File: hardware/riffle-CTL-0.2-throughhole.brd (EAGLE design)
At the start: 36.8 x 18 mm, 14 parts, among them J2 AYZ0202

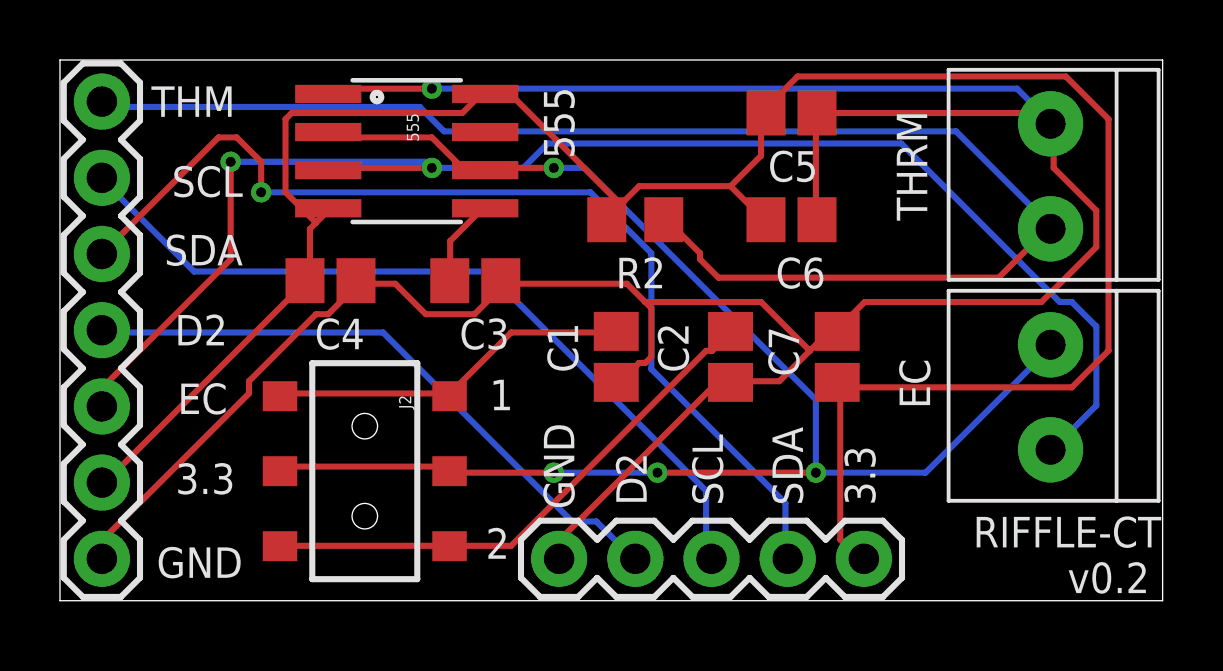
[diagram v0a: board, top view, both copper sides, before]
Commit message: update
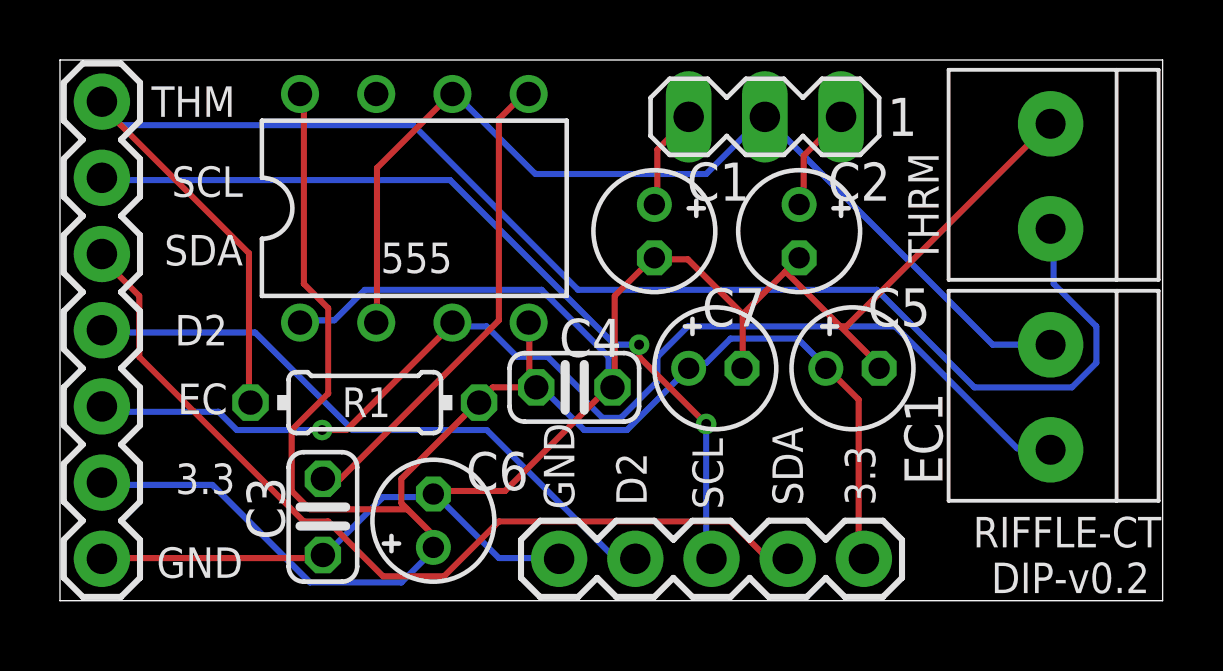
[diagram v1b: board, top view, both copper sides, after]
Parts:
- removed 555: NE555D, SparkFun-AnalogIC:SO08@1
- removed J2: AYZ0202, SparkFunNew:AYZ0202
- removed R2: 10k, rcl:R0805
- added IC1: LM555N, linear:DIL08
- added R1: 10k, resistor:0204/7
- added SV1: (no value), con-lstb:MA03-1
- C1, C7: value 1uF -> 10µ; device resistor:C0805 -> resistor:E1,8-4
- C2: value .1uF -> .1; device resistor:C0805 -> resistor:E1,8-4
- C3: value .01u -> 0.01µ; device resistor:C0805 -> resistor:C025-024X044
- C4: value 100n -> 0.1µ; device resistor:C0805 -> resistor:C025-024X044
- C5: value 100n -> .1µ; device resistor:C0805 -> resistor:E1,8-4
- C6: value .1uF -> 1u; device resistor:C0805 -> resistor:E1,8-4
- moved C6 15.6 mm to (12.4, 2.67), turned to 90 degrees
- moved C3 9.37 mm to (8.76, 2.79), turned to 90 degrees
- moved C4 8.87 mm to (17.1, 7.11), turned to 0 degrees
- moved C5 8.75 mm to (26.4, 7.75), turned to 0 degrees
- moved C2 4.77 mm to (24.6, 12.3)
- moved C1 4.38 mm to (19.8, 12.3)
- moved C7 4.08 mm to (21.8, 7.75), turned to 0 degrees
- renumbered EC to EC1
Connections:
- removed net N$2: 555.5, C3.2
- removed net N$6: C2.1, J2.3, J2.6
- removed net N1: 555.2, 555.6, EC1.1, J2.2, J2.5
- removed net VDD2: C1.1, J2.1, J2.4
- new net N$1: C1.+, SV1.3
- new net N$3: EC1.1, IC1.2, IC1.6, SV1.2
- new net N$4: C2.+, SV1.1
- new net N$7: C3.2, IC1.5
- net EC: now also IC1.3; no longer 555.3
- net GND: now also C1.-, C2.-, C4.2, C5.-, C6.-, C7.-, IC1.1; no longer 555.1, C1.2, C2.2, C4.1, C5.1, C6.1, C7.1
- net THRM: now also R1.1; no longer R2.1
- net VCC: now also C4.1, C5.+, C6.+, C7.+, IC1.4, IC1.8, R1.2; no longer 555.4, 555.8, C4.2, C5.2, C6.2, C7.2, R2.2
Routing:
- net N1: track 50.2 -> 0.00 mm, vias 4 -> 0
- net N$3: track 0.00 -> 33.6 mm
- net GND: track 97.5 -> 64.7 mm, vias 1 -> 0
- net N$6: track 18.0 -> 0.00 mm
- net N$7: track 0.00 -> 16.1 mm
- net VCC: track 75.5 -> 60.9 mm
- net VDD2: track 12.2 -> 0.00 mm
- net EC: track 50.0 -> 38.4 mm, vias 2 -> 1
- net THRM: track 48.0 -> 54.7 mm
- net SDA: track 34.2 -> 29.8 mm, vias 1 -> 0
- net N$4: track 0.00 -> 3.58 mm
- net N$1: track 0.00 -> 3.45 mm
- net N$2: track 2.93 -> 0.00 mm
- net SCL: track 26.9 -> 28.5 mm, vias 0 -> 2
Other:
- board text added: "DIP-v0.2"
- board text removed: "1"
- board text removed: "2"
- board text removed: "RIFFLE-CT-0.2"
- board text removed: "conductivity + temperature"
- board text removed: "v0.2"
